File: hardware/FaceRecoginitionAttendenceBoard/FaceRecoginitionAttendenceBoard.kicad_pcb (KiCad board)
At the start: 2 copper layers, 60 x 50 mm, 6 parts, among them J1 Barrel_Jack_Switch, J2 PROGRAMMING CONNECTOR, U1 ESP32-CAM

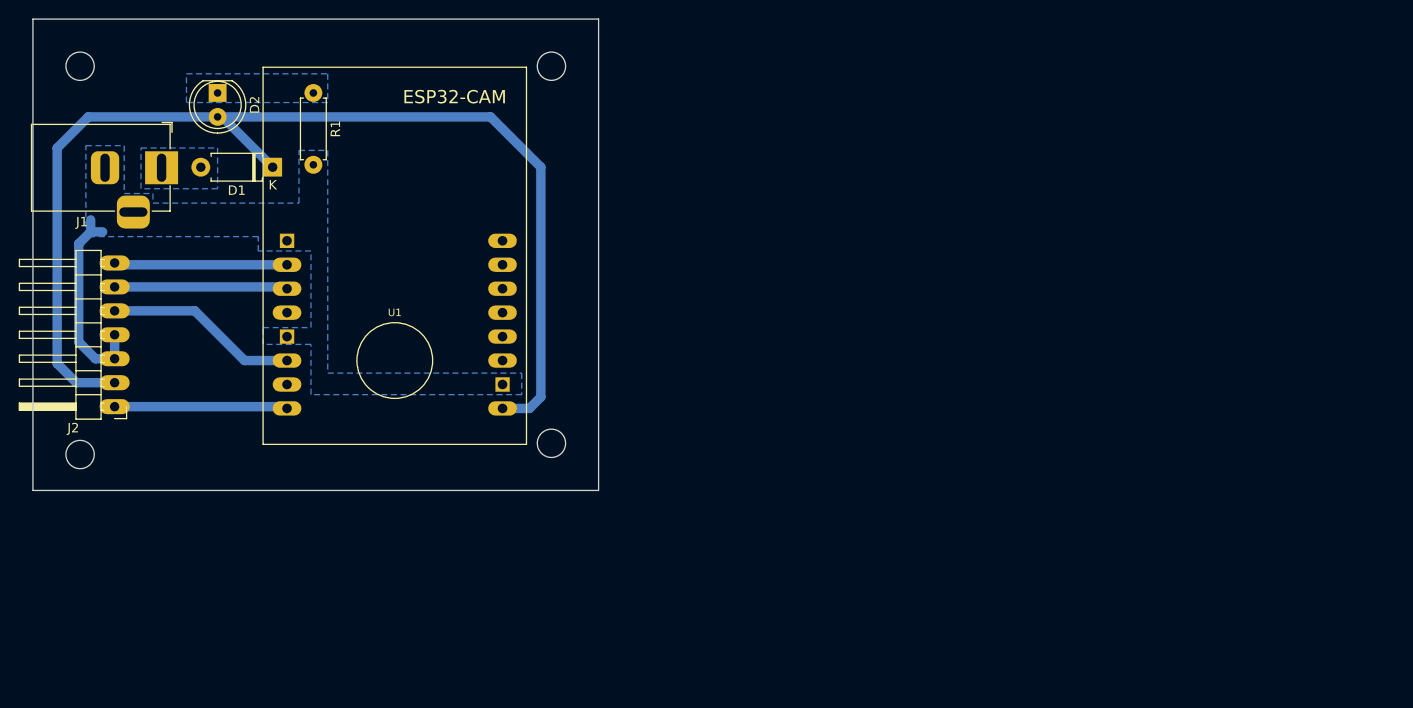
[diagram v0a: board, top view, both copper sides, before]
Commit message: Updated hardware design
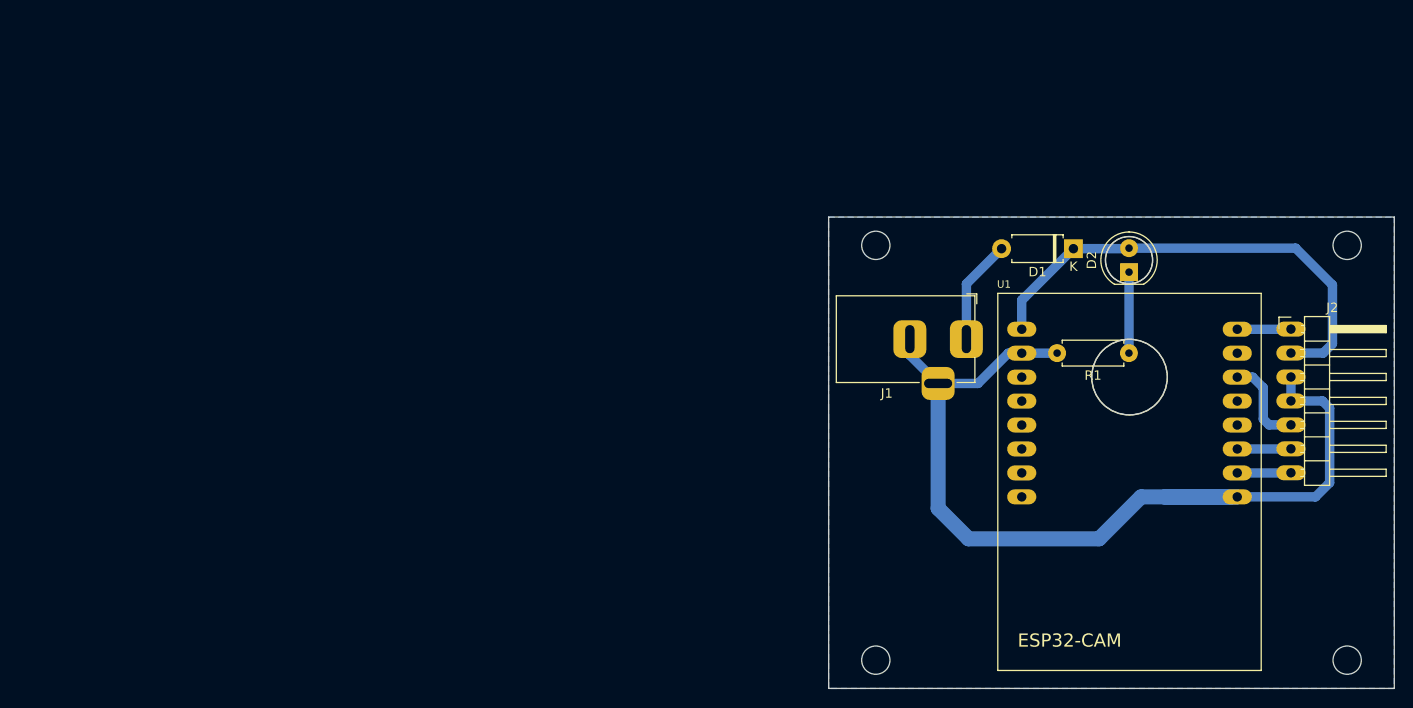
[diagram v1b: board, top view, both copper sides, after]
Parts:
- moved J2 125.0 mm to (156.3, 56.8), turned to 0 degrees
- moved D2 98.5 mm to (139.1, 50.8), turned to 90 degrees
- moved R1 90.8 mm to (139.1, 59.3), turned to 180 degrees
- moved J1 87.3 mm to (121.8, 57.9)
- moved D1 85.4 mm to (133.2, 48.3)
- moved U1 78.8 mm to (139.1, 67.0), turned to 180 degrees
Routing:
- net GND: track 23.6 -> 101.1 mm
- net +5V: track 121.7 -> 51.0 mm
- net UART_TX: track 18.4 -> 5.70 mm
- net +3.3V: track 18.1 -> 5.70 mm
- net UART_RX: track 18.1 -> 5.70 mm
- net Net-(D1-A): track 0.00 -> 11.1 mm
- net GPIO_0: track 20.5 -> 9.74 mm
- net Net-(D2-K): track 0.00 -> 8.59 mm
- added copper zone on B.Cu, net (none)
- removed copper zone on B.Cu, net GND
- removed copper zone on B.Cu, net Net-(D1-A)
- removed copper zone on B.Cu, net Net-(D2-K)
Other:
- outline, holes or cut-outs redrawn
